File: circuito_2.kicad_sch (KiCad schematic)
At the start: 25 parts, among them U1 TL081, U2 TL081, U3 TL081

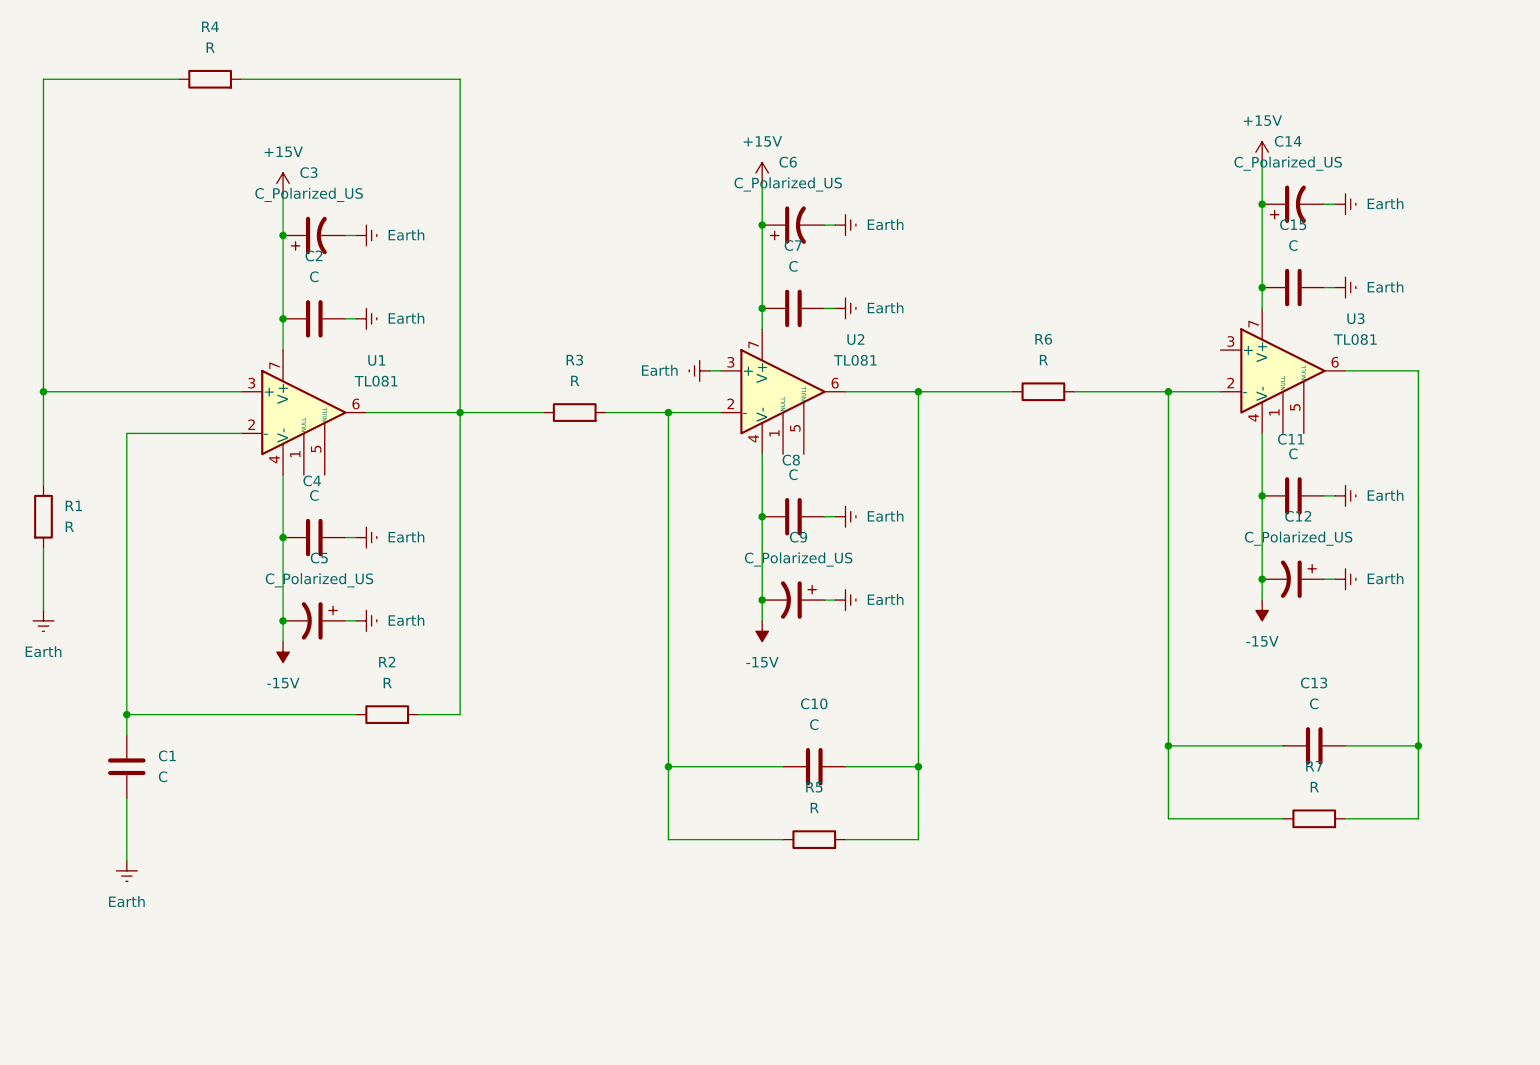
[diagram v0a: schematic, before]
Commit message: Reorganização dos esquemáticos em pages.
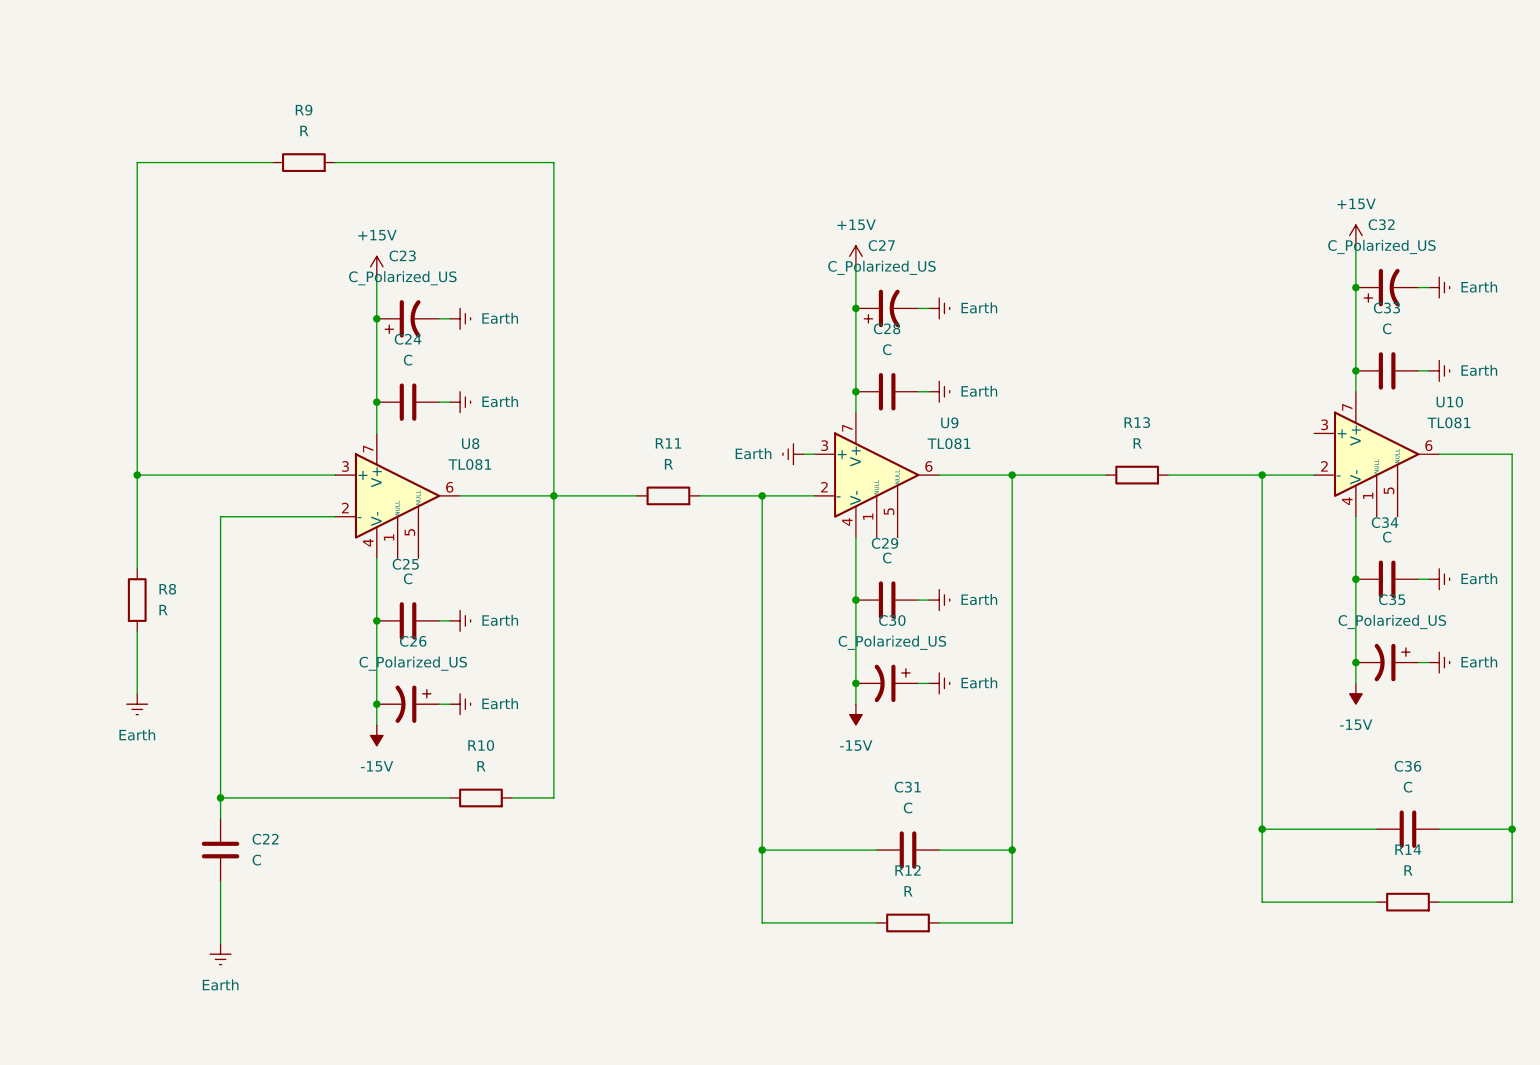
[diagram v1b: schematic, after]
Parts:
- removed C1, C10, C11, C13, C15, C2, C4, C7, C8: C, symbol Device:C
- removed C12, C14, C3, C5, C6, C9: C_Polarized_US, symbol Device:C_Polarized_US
- removed R1, R2, R3, R4, R5, R6, R7: R, symbol Device:R
- removed U1, U2, U3: TL081, symbol Amplifier_Operational:TL081
- added C22, C24, C25, C28, C29, C31, C33, C34, C36: C, symbol Device:C
- added C23, C26, C27, C30, C32, C35: C_Polarized_US, symbol Device:C_Polarized_US
- added R10, R11, R12, R13, R14, R8, R9: R, symbol Device:R
- added U10, U8, U9: TL081, symbol Amplifier_Operational:TL081
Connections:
- net +15V: now also C23.1, C24.1, C27.1, C28.1, C32.1, C33.1, U10.7 (V+), U8.7 (V+), U9.7 (V+)
- net -15V: now also C25.1, C26.2, C29.1, C30.2, C34.1, C35.2, U10.4 (V-), U8.4 (V-), U9.4 (V-)
- net Earth: now also C22.2, C23.2, C24.2, C25.2, C26.1, C27.2, C28.2, C29.2, C30.1, C32.2, C33.2, C34.2, C35.1, R8.2, U9.3 (+)
- new net: C22.1, R10.1, U8.2 (-)
- new net: C36.1, R13.2, R14.1, U10.2 (-)
- new net: C36.2, R14.2, U10.6
- new net: C31.2, R12.2, R13.1, U9.6
- new net: R8.1, R9.1, U8.3 (+)
- new net: R10.2, R11.1, R9.2, U8.6
- new net: C31.1, R11.2, R12.1, U9.2 (-)

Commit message: Footprints parcialmente adicionados.
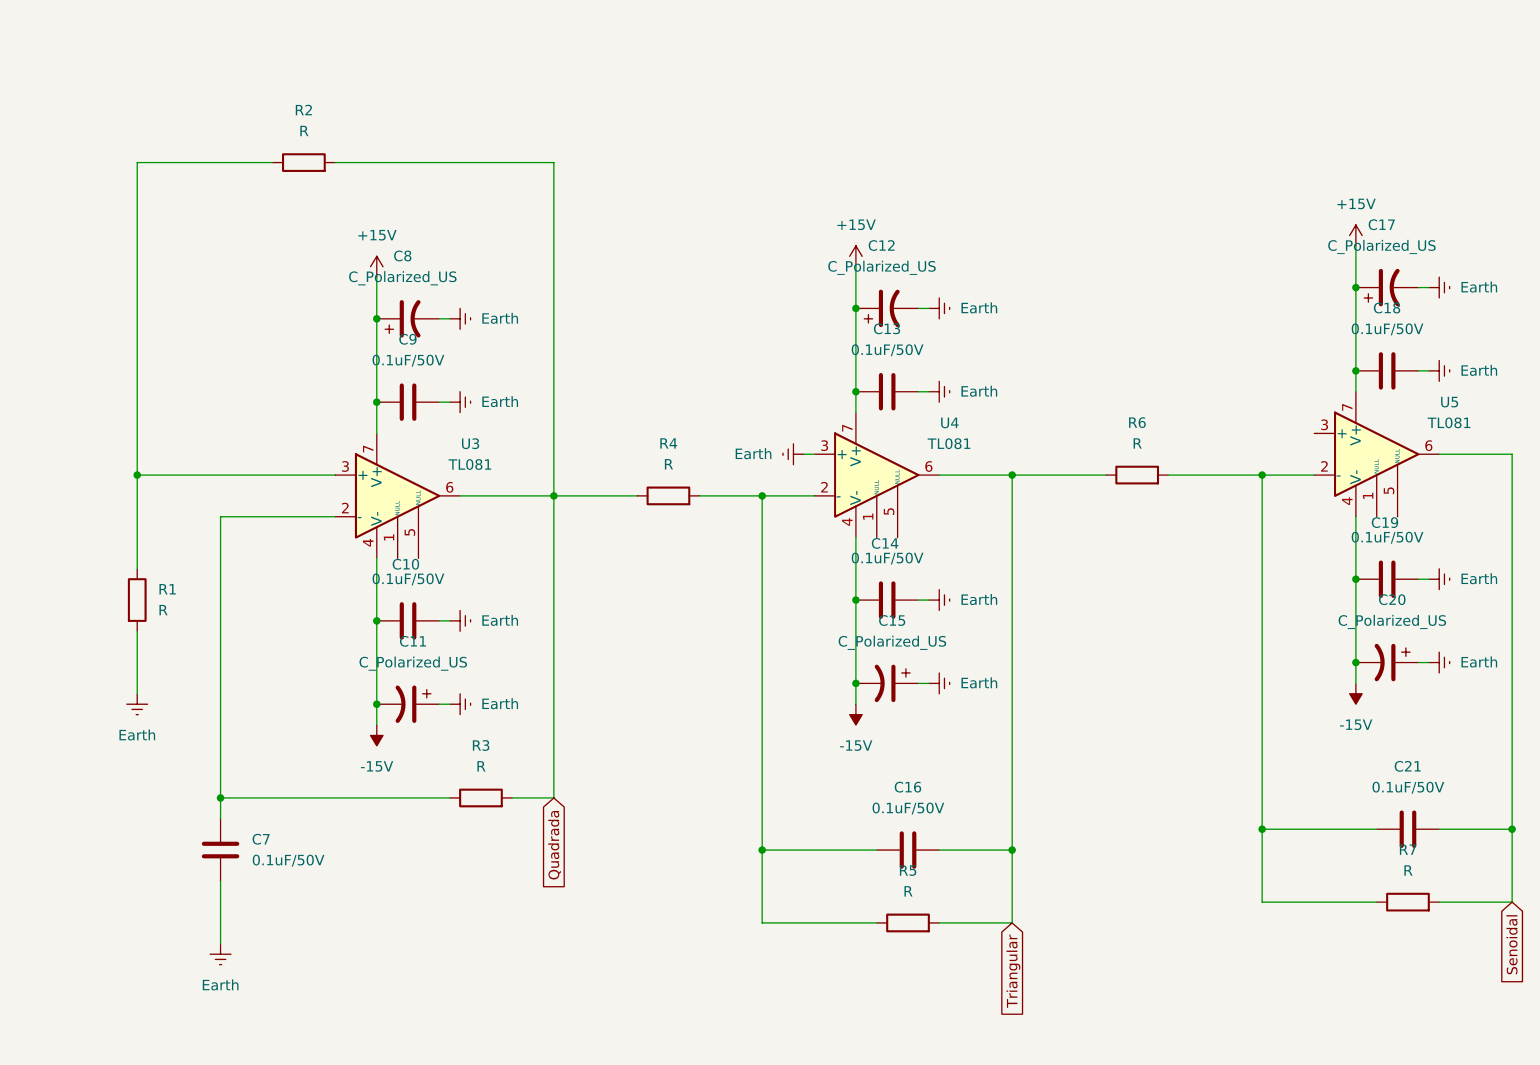
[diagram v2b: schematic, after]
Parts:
- C10: renamed from C25; value C -> 0.1uF/50V; footprint (none) -> Capacitor_THT:C_Disc_D3.8mm_W2.6mm_P2.50mm
- C13: renamed from C28; value C -> 0.1uF/50V; footprint (none) -> Capacitor_THT:C_Disc_D3.8mm_W2.6mm_P2.50mm
- C14: renamed from C29; value C -> 0.1uF/50V; footprint (none) -> Capacitor_THT:C_Disc_D3.8mm_W2.6mm_P2.50mm
- C16: renamed from C31; value C -> 0.1uF/50V; footprint (none) -> Capacitor_THT:C_Disc_D3.8mm_W2.6mm_P2.50mm
- C18: renamed from C33; value C -> 0.1uF/50V; footprint (none) -> Capacitor_THT:C_Disc_D3.8mm_W2.6mm_P2.50mm
- C19: renamed from C34; value C -> 0.1uF/50V; footprint (none) -> Capacitor_THT:C_Disc_D3.8mm_W2.6mm_P2.50mm
- C21: renamed from C36; value C -> 0.1uF/50V; footprint (none) -> Capacitor_THT:C_Disc_D3.8mm_W2.6mm_P2.50mm
- C7: renamed from C22; value C -> 0.1uF/50V; footprint (none) -> Capacitor_THT:C_Disc_D3.8mm_W2.6mm_P2.50mm
- C9: renamed from C24; value C -> 0.1uF/50V; footprint (none) -> Capacitor_THT:C_Disc_D3.8mm_W2.6mm_P2.50mm
- renumbered C26 to C11, C27 to C12, C30 to C15, C32 to C17, C35 to C20, C23 to C8, R8 to R1, R9 to R2, R10 to R3, R11 to R4, R12 to R5, R13 to R6, R14 to R7, U8 to U3, U9 to U4, U10 to U5
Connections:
- net Senoidal: now reaches C21.2, R7.2, U5.6
- net Triangular: now reaches C16.2, R5.2, R6.1, U4.6
- net Quadrada: now reaches R2.2, R3.2, R4.1, U3.6
